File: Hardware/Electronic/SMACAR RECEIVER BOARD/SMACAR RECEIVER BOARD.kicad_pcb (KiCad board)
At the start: 2 copper layers, 11 parts, among them J1 M04POLAR, J2 USB_C_Receptacle_USB2.0_14P, U1 ESP32-S3-DevKitC, U2 TVS0500DRV, U3 TVS0500DRV

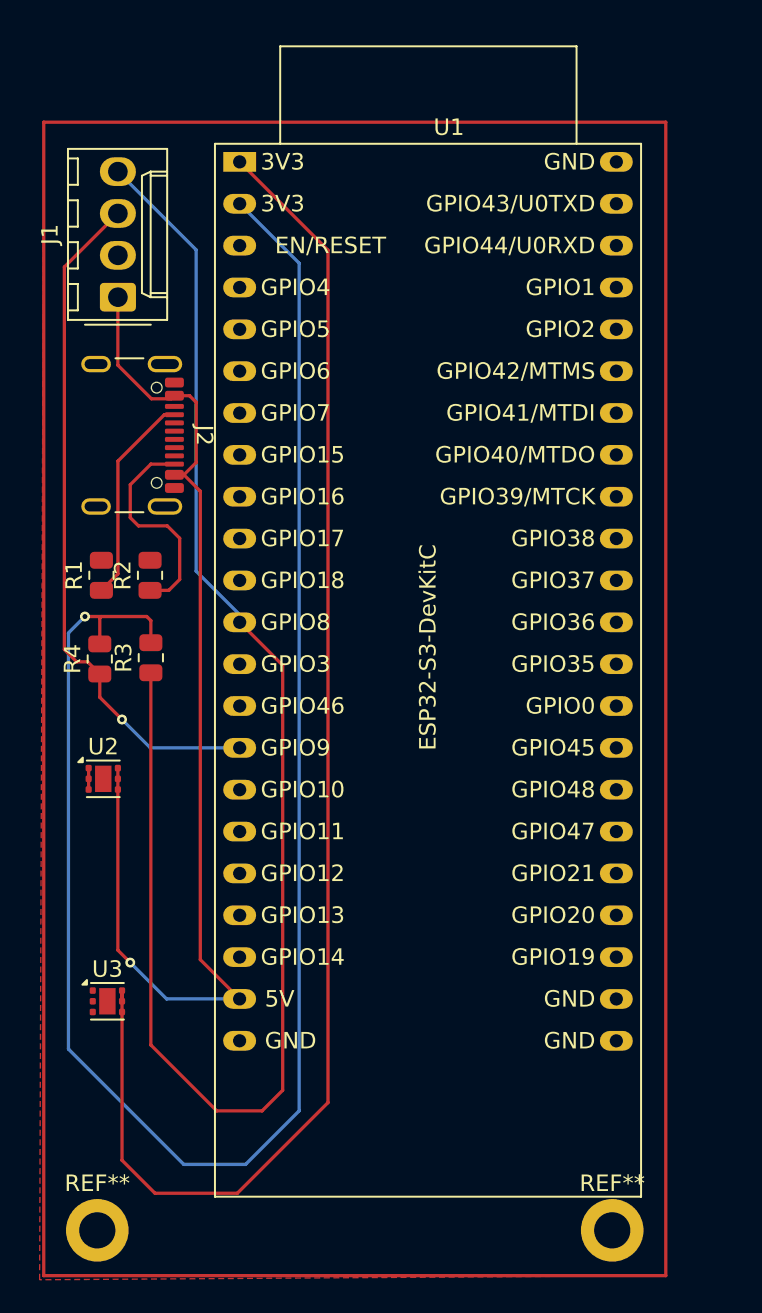
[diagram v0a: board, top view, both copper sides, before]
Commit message: V1.0 Revision
Revision for V1.0 of the project. Includes production files for JLCPCB. Some footprints and schematic symbols were changed.
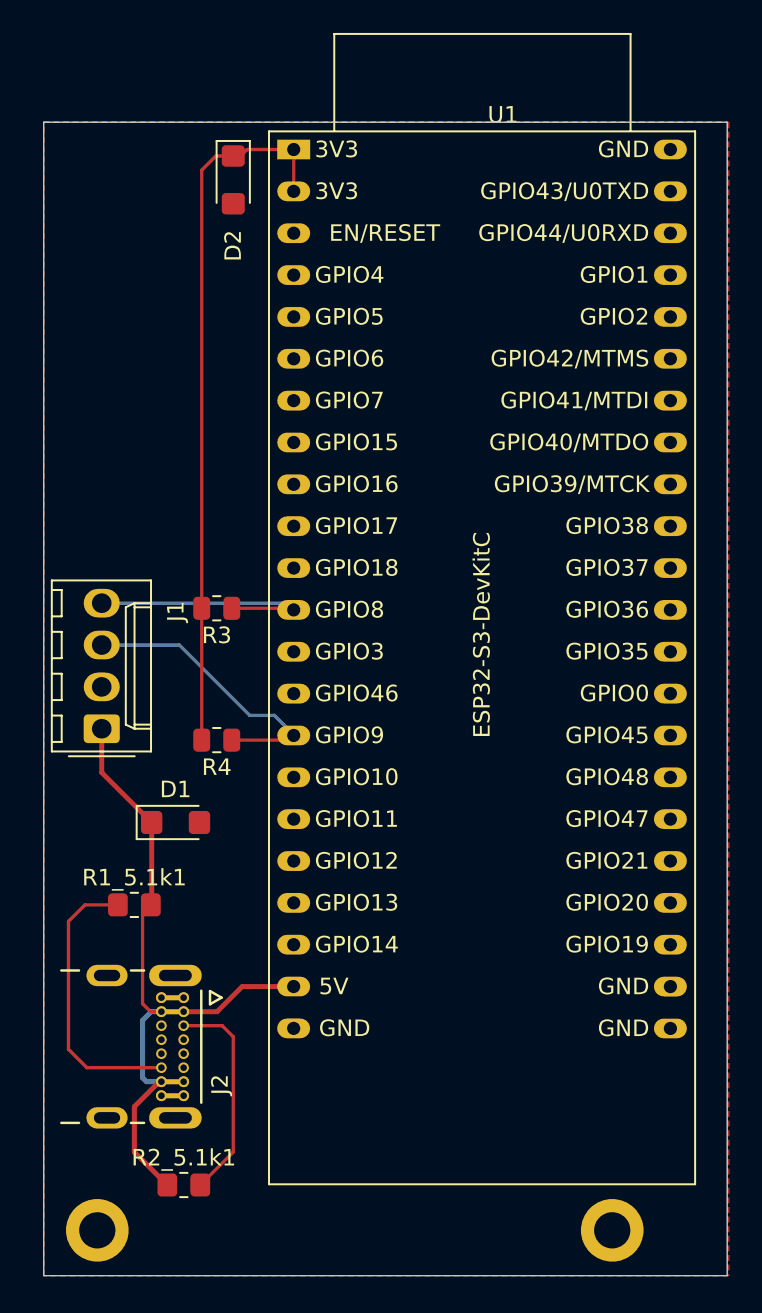
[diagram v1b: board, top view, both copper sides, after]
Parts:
- removed R1, R2: 470R_0805_350mW, Resistor_SMD:R_0805_2012Metric
- removed U2, U3: TVS0500DRV, Package_SON:WSON-6-1EP_2x2mm_P0.65mm_EP1x1.6mm
- added D1: SMF33A, Diode_SMD:D_SMF, F.Cu at (131.5, 92.0)
- added D2: SMF33A, Diode_SMD:D_SMF, F.Cu at (135.0, 53.0)
- added R1_5.1k1: 470R_0805_350mW, Resistor_SMD:R_0805_2012Metric_Pad1.20x1.40mm_HandSolder, F.Cu at (129.0, 97.0)
- added R2_5.1k1: 470R_0805_350mW, Resistor_SMD:R_0805_2012Metric_Pad1.20x1.40mm_HandSolder, F.Cu at (132.0, 114.0)
- J2: value USB_C_Receptacle_USB2.0_14P -> 2137160001; footprint Connector_USB:USB_C_Receptacle_GCT_USB4105-xx-A_16P_TopMnt_Horizontal -> XUNPU TYPEC-306DDW-ARP16:MOLEX_2137160001
- moved J2 37.3 mm to (124.3, 105.6)
- moved J1 26.2 mm to (127.0, 86.3)
- moved R4 8.64 mm to (134.0, 87.0), turned to 180 degrees
- moved R3 5.00 mm to (134.0, 79.0), turned to 180 degrees
- moved U1 3.37 mm to (138.7, 51.2)
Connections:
- J2 pad A8: (no net) -> unconnected-(J2-SBU1-PadA8)
- J2 pad B8: (no net) -> unconnected-(J2-SBU2-PadB8)
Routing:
- net Net-(D2-A1): track 194.5 -> 43.4 mm, vias 1 -> 0
- net SDA: track 92.7 -> 15.6 mm
- net 5V: track 68.1 -> 41.3 mm, vias 1 -> 0
- net SCL: track 41.7 -> 17.8 mm, vias 1 -> 0
- net Net-(J2-CC2): track 13.3 -> 17.3 mm
- net GND: track 1.30 -> 0.00 mm
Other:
- board outline added: 41.5 x 70 mm
